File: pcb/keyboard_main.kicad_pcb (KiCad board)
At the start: 2 copper layers, 81.5 x 32.3 mm, 17 parts

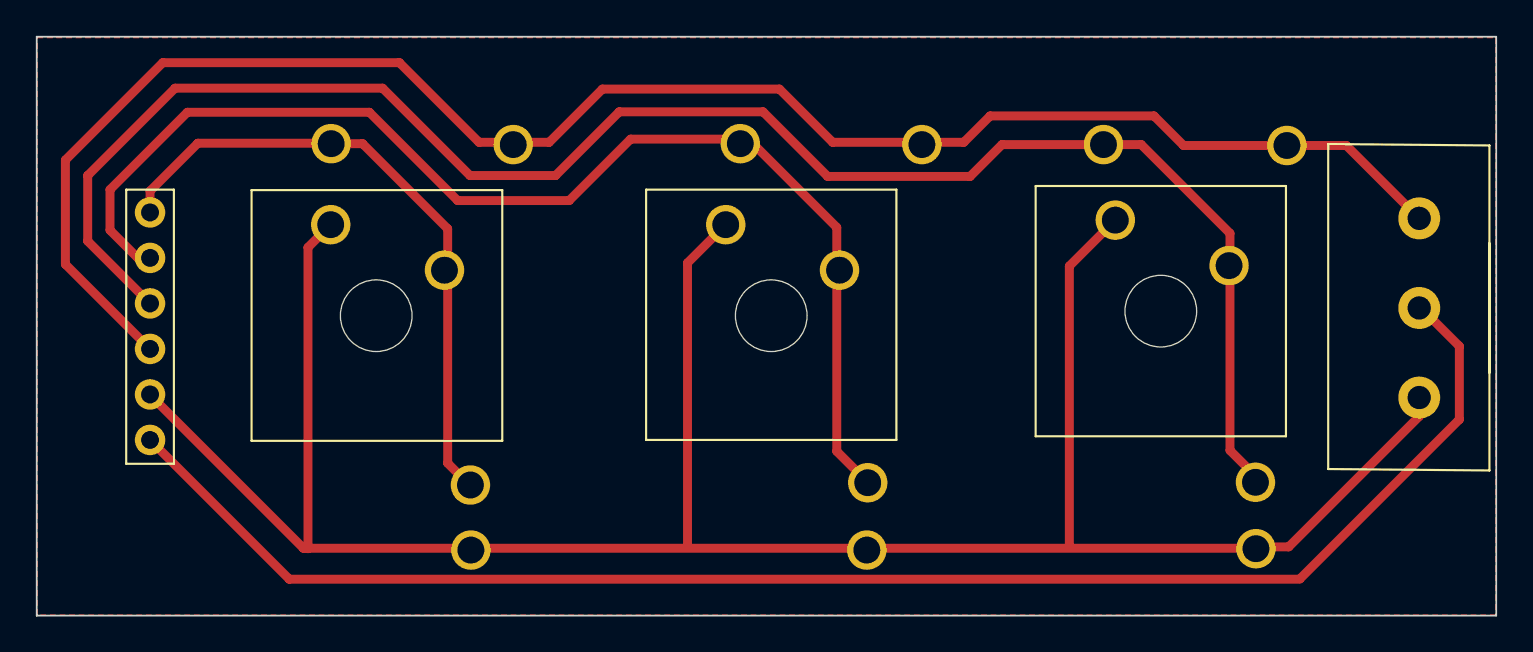
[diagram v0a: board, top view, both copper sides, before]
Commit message: Update pcb design
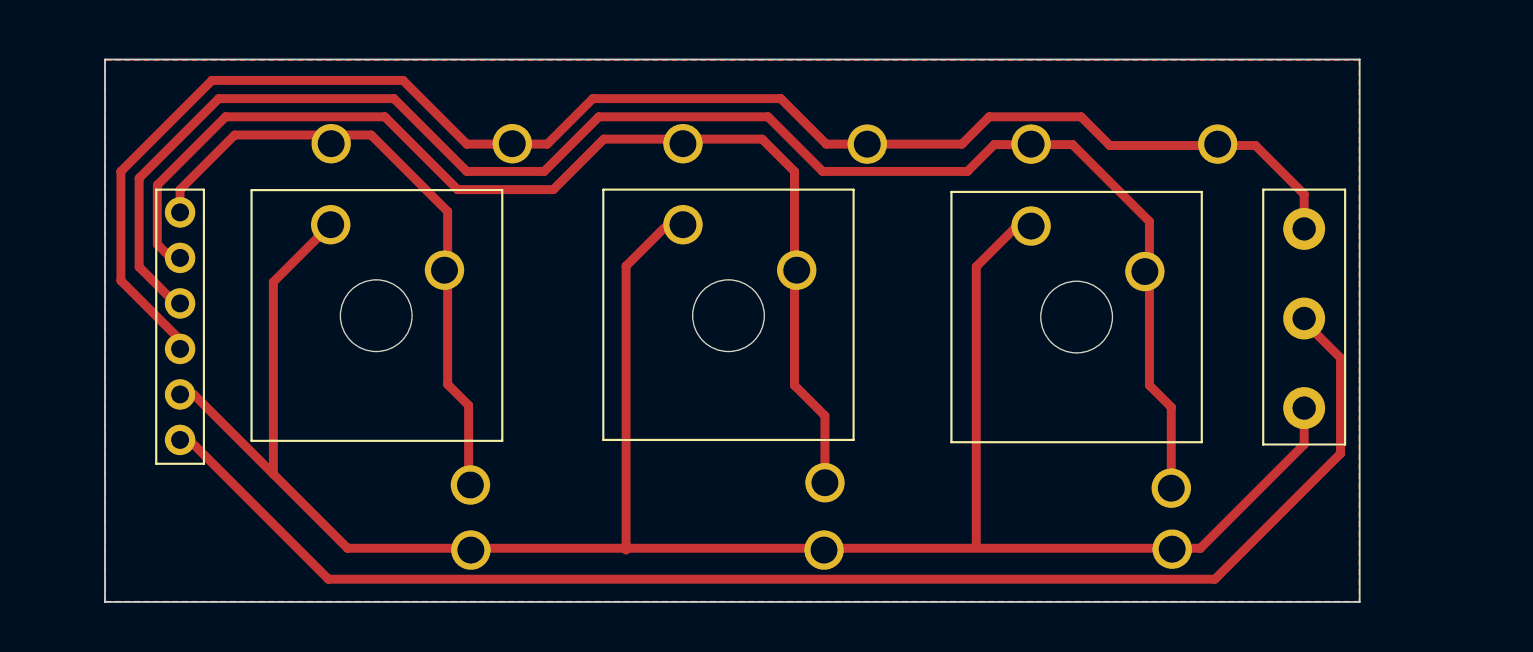
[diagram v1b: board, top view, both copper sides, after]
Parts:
- moved REF** 6.45 mm to (115.3, 47.8)
- moved ? 4.71 mm to (107.9, 52.2)
- moved REF** 4.71 mm to (100.1, 37.6)
- moved ? 4.67 mm to (108.0, 55.6)
- moved ? 4.04 mm to (100.1, 33.0)
- moved ? 3.86 mm to (110.5, 33.0)
- moved ? 3.20 mm to (80.6, 33.0)
- moved ? 3.05 mm to (90.9, 33.0)
- moved ? 2.39 mm to (88.6, 51.9)
- moved REF** 2.39 mm to (80.6, 37.5)
- moved ? 2.39 mm to (88.5, 55.7)
- moved REF** 1.68 mm to (52.6, 36.8)
- moved ? 0.07 mm to (71.1, 33.0)
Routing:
- net (no net): track 519.8 -> 476.1 mm
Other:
- board size 81.5 x 32.3 mm -> 70 x 30.3 mm
- board text added: "keyboard v2 @dybarsky"
- board text removed: "keyboard v1 @dybarsky"
